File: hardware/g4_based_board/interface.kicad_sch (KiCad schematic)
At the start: 26 parts, among them J1 USB_C_Receptacle_USB2.0, J2 Micro_SD_Card_Det1, Q1 NPN, Q2 NPN

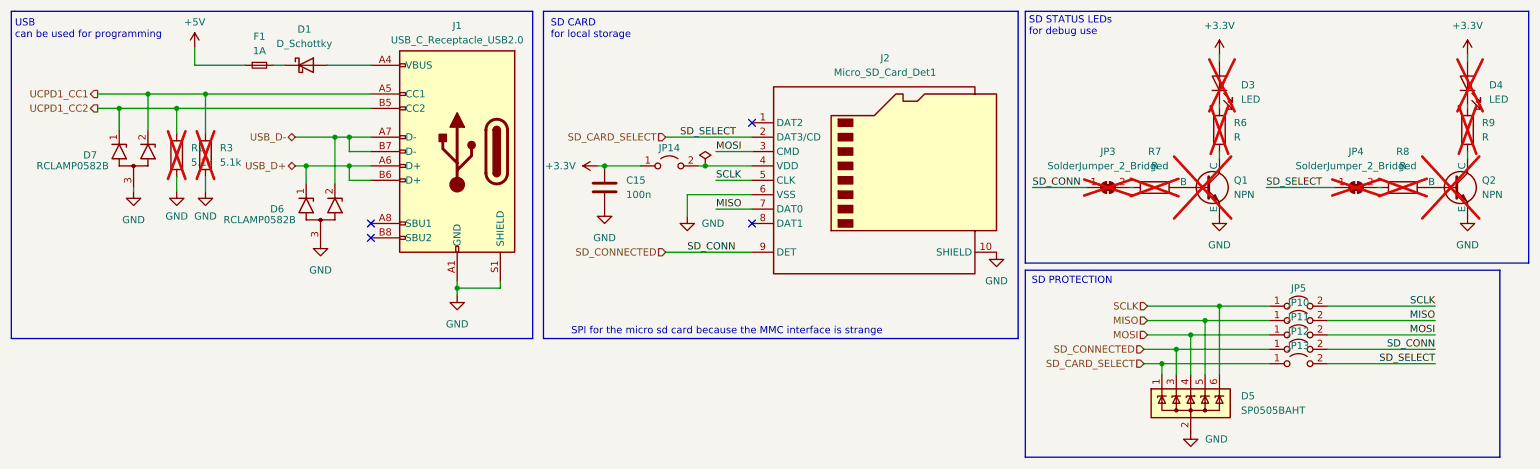
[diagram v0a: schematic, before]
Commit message: git thinks something changed in this file
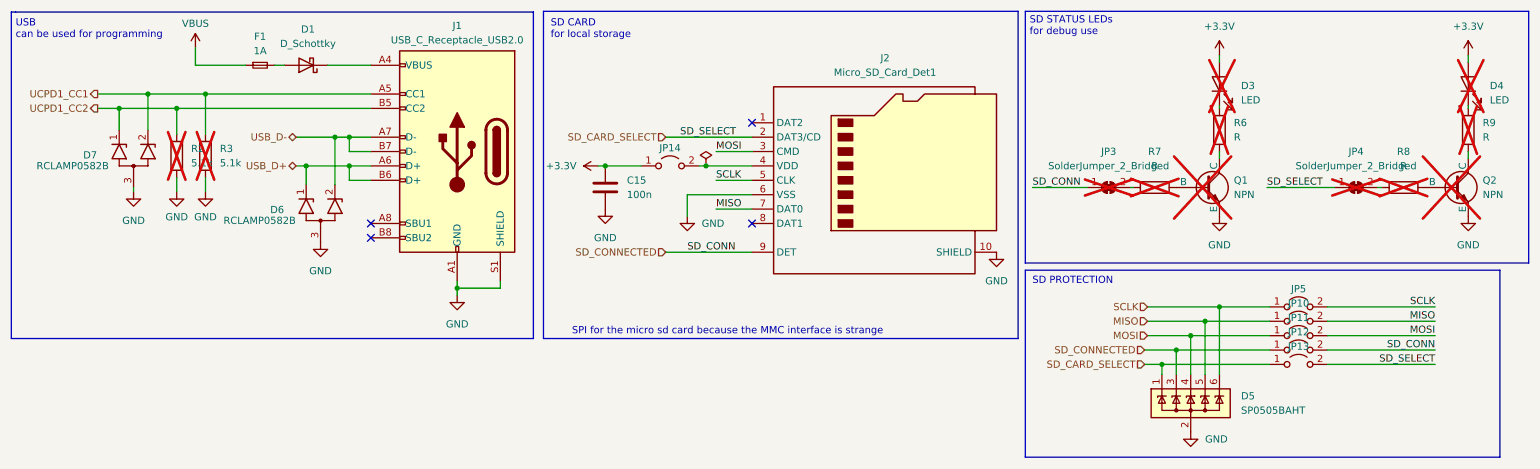
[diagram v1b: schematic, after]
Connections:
- net at J1.A4 (VBUS), J1.A9 (VBUS), J1.B4 (VBUS)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: now also D1.1 (K); no longer D1.2 (A)
- net at F1.2: now also D1.2 (A); no longer D1.1 (K)
- net +5V renamed VBUS
